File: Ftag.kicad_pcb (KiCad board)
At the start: 2 copper layers, 34.9 x 29.2 mm, 25 parts, among them P1 USB_OTG, P2 CONN_10X2, U1 FT232H, U2 TXB0108, X1 12 MHz

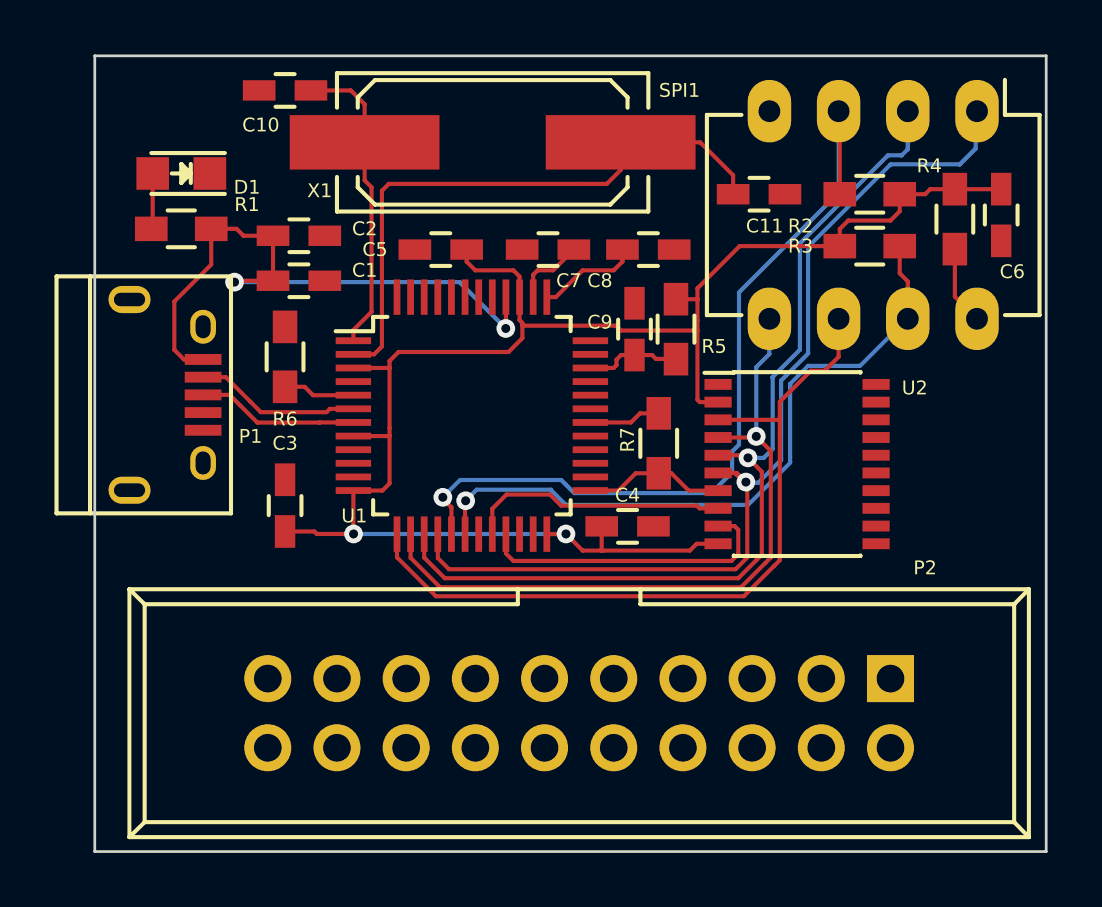
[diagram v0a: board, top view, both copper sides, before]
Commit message: Finished preliminary layout
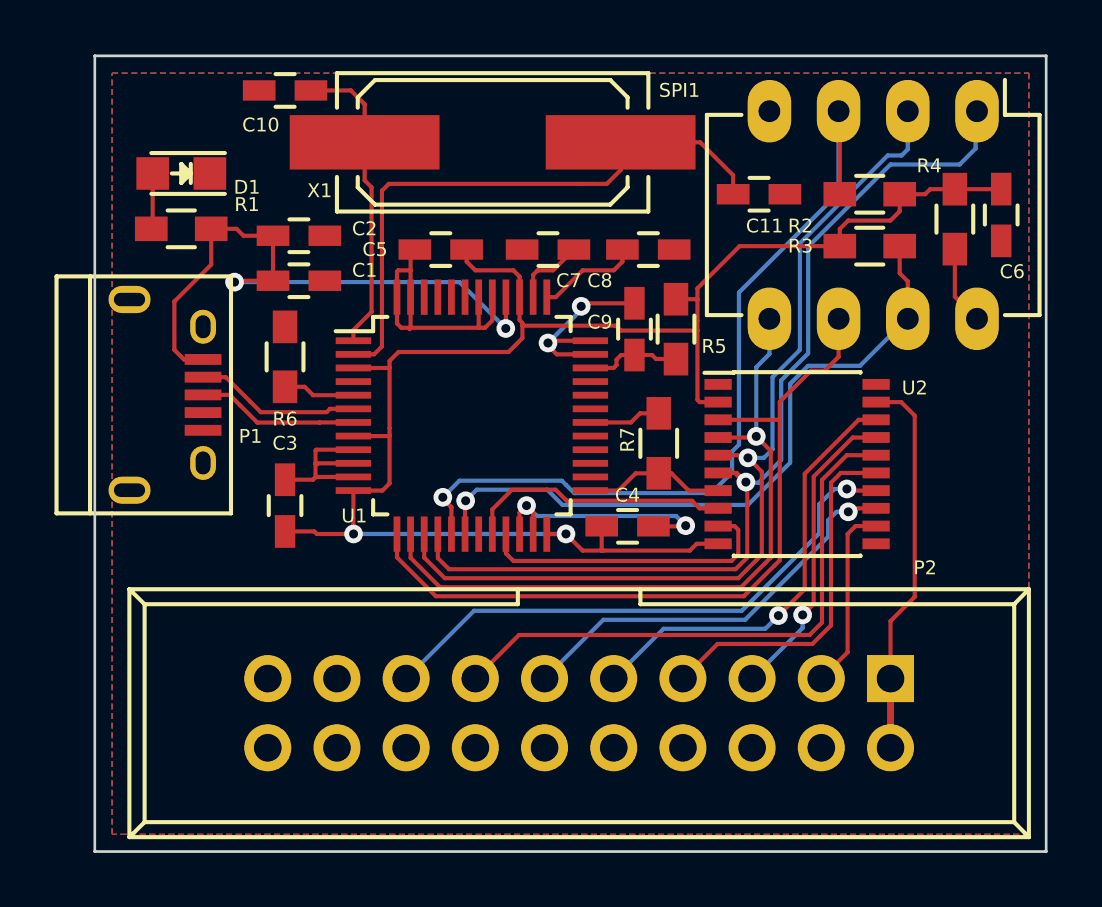
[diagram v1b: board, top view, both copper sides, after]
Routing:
- net GND: track 0.00 -> 34.6 mm, vias 0 -> 4
- net /SRST: track 0.00 -> 21.5 mm, vias 0 -> 1
- net /TDO: track 0.00 -> 21.2 mm
- net /TCK: track 0.00 -> 16.1 mm, vias 0 -> 1
- net /RTCK: track 0.00 -> 15.1 mm, vias 0 -> 1
- net /VCCIO: track 0.00 -> 14.2 mm
- net /TMS: track 0.00 -> 13.3 mm
- net /TDI: track 0.00 -> 11.2 mm, vias 0 -> 1
- net /TRST: track 0.00 -> 6.87 mm
- added copper zone on B.Cu, net GND
- added copper zone on F.Cu, net GND
